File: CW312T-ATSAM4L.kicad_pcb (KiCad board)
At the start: 2 copper layers, 58.7 x 53.7 mm, 30 parts, among them J1 614105150721, P1 PCIEx4 EDGE CONNECTOR, U1 ATSAM4LC2AA-AU

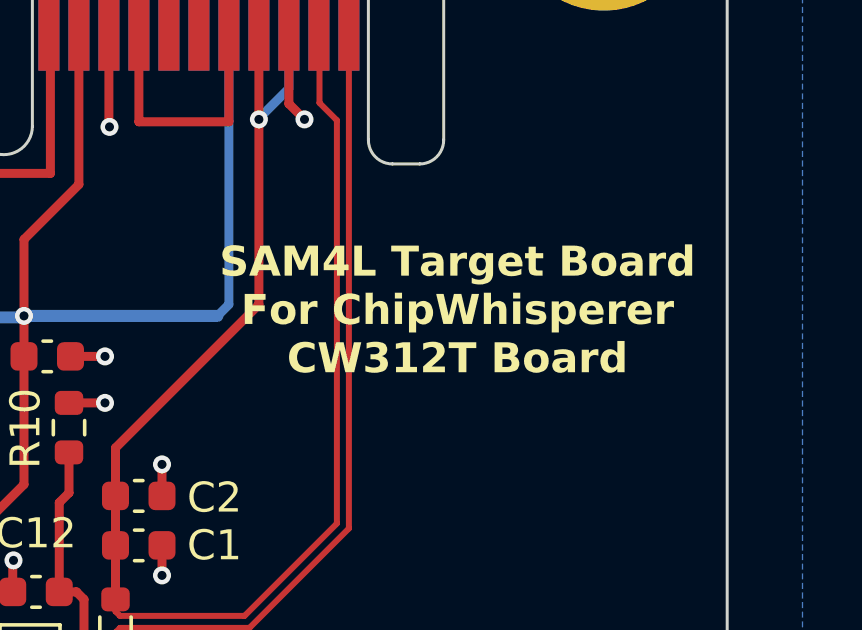
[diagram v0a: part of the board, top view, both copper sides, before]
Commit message: updated schematic, pcb, and production files - ready for review
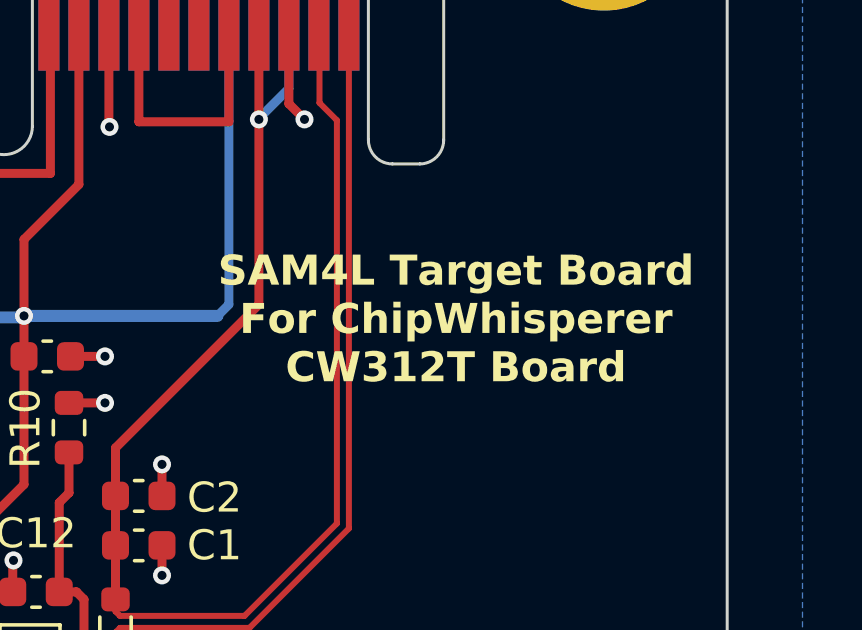
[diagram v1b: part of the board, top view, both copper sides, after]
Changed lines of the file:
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@@
 		(tags "resistor")
 		(property "Reference" "R9"
-			(at -0.075 -1.55 360)
+			(at -0.075 -1.55 0)
 			(layer "F.SilkS")
 			(effects
@@
 		)
 		(property "Value" "RES_10k_0603"
-			(at 0 1.43 360)
+			(at 0 1.43 0)
 			(layer "F.Fab")
 			(effects
@@
 		)
 		(fp_text user "${REFERENCE}"
-			(at 0 0 360)
+			(at 0 0 0)
 			(layer "F.Fab")
 			(effects
@@
 		(tags "resistor")
 		(property "Reference" "R2"
-			(at 2.525 0 360)
+			(at 2.525 0 0)
 			(layer "F.SilkS")
 			(effects
@@
 		)
 		(property "Value" "RES_47k_0603"
-			(at 0 1.43 360)
+			(at 0 1.43 0)
 			(layer "F.Fab")
 			(effects
@@
 		)
 		(fp_text user "${REFERENCE}"
-			(at 0 0 360)
+			(at 0 0 0)
 			(layer "F.Fab")
 			(effects
@@
 		(sheetname "Root")
 		(sheetfile "CW312T-ATSAM4L.kicad_sch")
-		(attr smd)
+		(attr smd dnp)
 		(fp_line
 			(start -0.14058 -0.51)
@@
 		(tags "capacitor")
 		(property "Reference" "C2"
-			(at 2.525 0.06 360)
+			(at 2.525 0.06 0)
 			(layer "F.SilkS")
 			(effects
@@
 		)
 		(property "Value" "CAP_2u2_6.3V_0603"
-			(at 0 1.43 360)
+			(at 0 1.43 0)
 			(layer "F.Fab")
 			(effects
@@
 		)
 		(fp_text user "${REFERENCE}"
-			(at 0 0 360)
+			(at 0 0 0)
 			(layer "F.Fab")
 			(effects
@@
 		(sheetname "Root")
 		(sheetfile "CW312T-ATSAM4L.kicad_sch")
-		(attr through_hole)
+		(attr through_hole dnp)
 		(fp_line
 			(start -2.85 -1.38)
@@
 		(tags "capacitor")
 		(property "Reference" "C1"
-			(at -2.525 0 360)
+			(at -2.525 0 0)
 			(layer "F.SilkS")
 			(effects
@@
 		)
 		(property "Value" "CAP_100n_10V_0603"
-			(at 0 1.43 360)
+			(at 0 1.43 0)
 			(layer "F.Fab")
 			(effects
@@
 		)
 		(fp_text user "${REFERENCE}"
-			(at 0 0 360)
+			(at 0 0 0)
 			(layer "F.Fab")
 			(effects
@@
 		(tags "capacitor")
 		(property "Reference" "C12"
-			(at 0 1.95 360)
+			(at 0 1.95 0)
 			(layer "F.SilkS")
 			(effects
@@
 		)
 		(property "Value" "CAP_2u2_6.3V_0603"
-			(at 0 1.43 360)
+			(at 0 1.43 0)
 			(layer "F.Fab")
 			(effects
@@
 		)
 		(fp_text user "${REFERENCE}"
-			(at 0 0 360)
+			(at 0 0 0)
 			(layer "F.Fab")
 			(effects
@@
 		(tags "resistor")
 		(property "Reference" "R7"
-			(at -2.4 -0.1 360)
+			(at -2.4 -0.1 0)
 			(layer "F.SilkS")
 			(effects
@@
 		)
 		(property "Value" "RES_1k5_0603"
-			(at 0 1.43 360)
+			(at 0 1.43 0)
 			(layer "F.Fab")
 			(effects
@@
 		)
 		(fp_text user "${REFERENCE}"
-			(at 0 0 360)
+			(at 0 0 0)
 			(layer "F.Fab")
 			(effects
@@
 		(tags "LQFP QFP")
 		(property "Reference" "U1"
-			(at 4.300001 4.5375 360)
+			(at 4.300001 4.5375 0)
 			(layer "F.SilkS")
 			(effects
@@
 		)
 		(property "Value" "ATSAM4LC2AA-AU"
-			(at 0 5.85 360)
+			(at 0 5.85 0)
 			(layer "F.Fab")
 			(effects
@@
 		)
 		(fp_text user "${REFERENCE}"
-			(at 0 0 360)
+			(at 0 0 0)
 			(layer "F.Fab")
 			(effects
@@
 		(tags "capacitor")
 		(property "Reference" "C10"
-			(at 2.975 -0.05 360)
+			(at 2.975 -0.05 0)
 			(layer "F.SilkS")
 			(effects
@@
 		)
 		(property "Value" "CAP_100n_10V_0603"
-			(at 0 1.43 360)
+			(at 0 1.43 0)
 			(layer "F.Fab")
 			(effects
@@
 		)
 		(fp_text user "${REFERENCE}"
-			(at 0 0 360)
+			(at 0 0 0)
 			(layer "F.Fab")
 			(effects
@@
 		(tags "capacitor")
 		(property "Reference" "C3"
-			(at -2.45 0 360)
+			(at -2.45 0 0)
 			(layer "F.SilkS")
 			(effects
@@
 		)
 		(property "Value" "CAP_47p_50V_0603"
-			(at 0 1.43 360)
+			(at 0 1.43 0)
 			(layer "F.Fab")
 			(effects
@@
 		(sheetname "Root")
 		(sheetfile "CW312T-ATSAM4L.kicad_sch")
-		(attr smd)
+		(attr smd dnp)
 		(fp_line
 			(start -0.140581 0.51)
@@
 		)
 		(fp_text user "${REFERENCE}"
-			(at 0 0 360)
+			(at 0 0 0)
 			(layer "F.Fab")
 			(effects
@@
 	)
 	(gr_text "SAM4L Target Board \nFor ChipWhisperer \nCW312T Board"
-		(at 162.2 78.8 0)
+		(at 162.15 79.1 0)
 		(layer "F.SilkS")
 		(effects
@@
 		(polygon
 			(pts
-				(xy 110.65 55.3) (xy 173.7 55.3) (xy 173.7 114.15) (xy 173.7 114.15) (xy 110.65 114.15)
+				(xy 110.65 55.3) (xy 173.7 55.3) (xy 173.7 114.15) (xy 110.65 114.15)
 			)
 		)
